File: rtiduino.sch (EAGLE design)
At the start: 144 parts, among them J1 DCJ0202, J2 3.5MM-JACK, J3 2.5MM-JACKPRO, J4 USB PROG, Q2 16MHz, U1 ATMEGA2560AU, U10 AQV252G, U11 AQV252G, U12 AQV252G, U13 AQV252G, U14 AQV252G, U15 AQV252G, U16 AQV252G, U17 AQV252G, U2 FT232RL, U20 AQV252G, U21 AQV252G, U22 AQV252G, U23 AQV252G, U24 AQV252G, U25 AQV252G, U26 AQV252G, U27 AQV252G, U3 LM2594HVM-5.0, U30 AQV252G, U31 AQV252G, U32 AQV252G, U33 AQV252G, U34 AQV252G, U35 AQV252G, U36 AQV252G, U37 AQV252G, U4 FT232RL, U5 FOD852, U6 LED-DRIVER, U7 FOD852

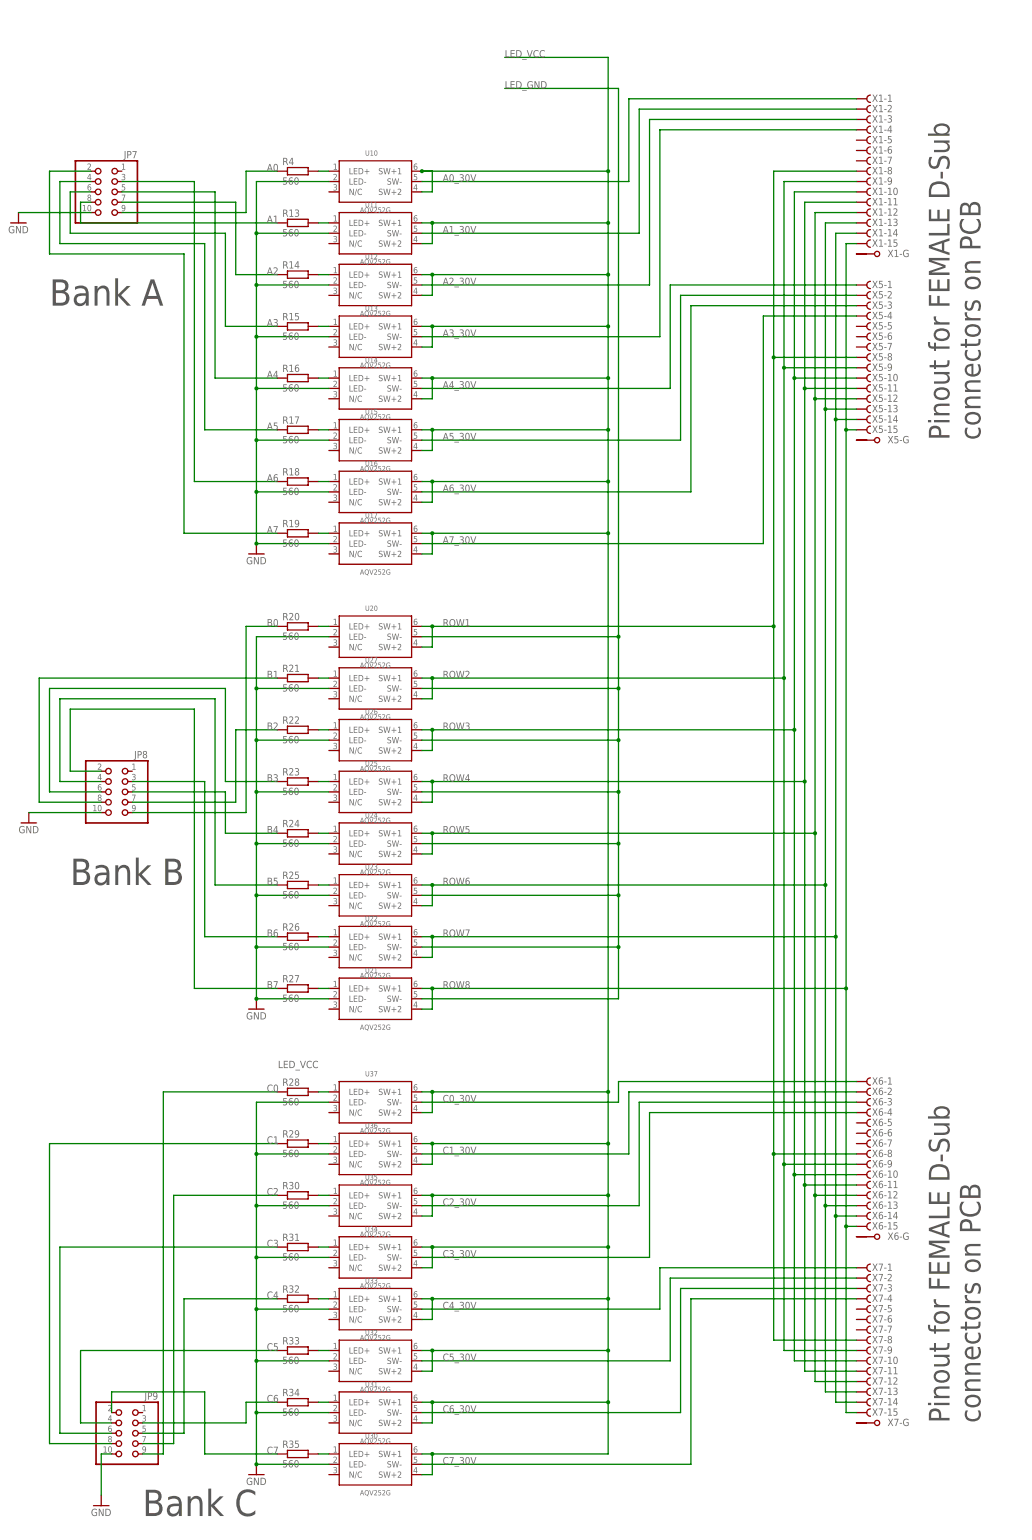
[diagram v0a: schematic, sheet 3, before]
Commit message: UPDATES
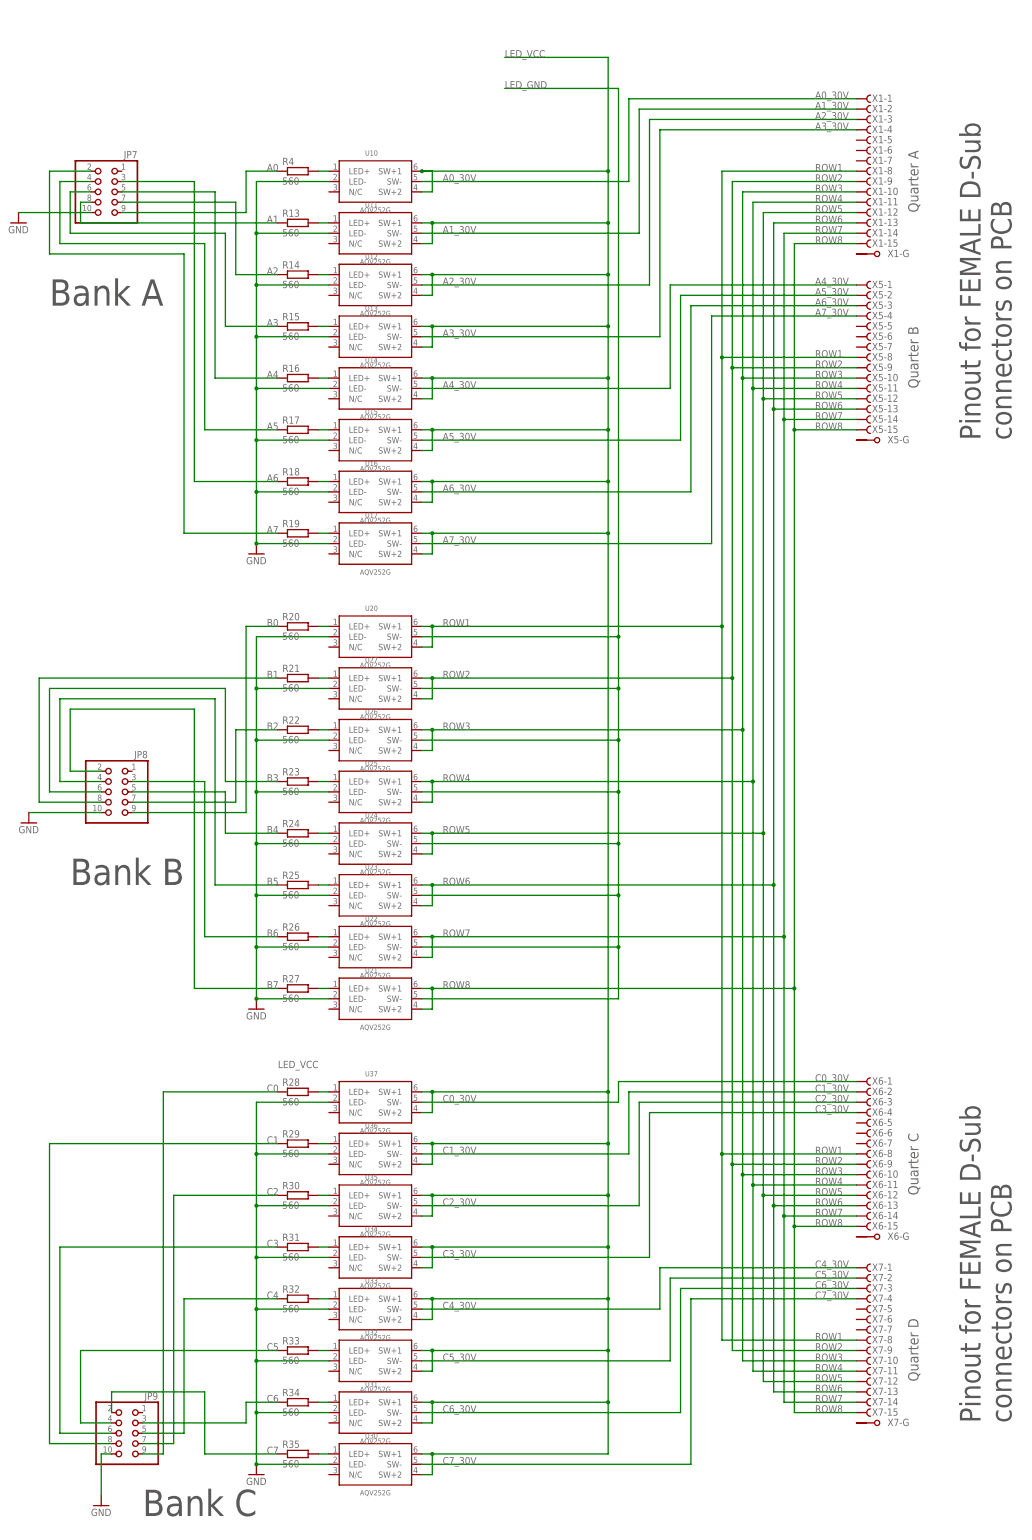
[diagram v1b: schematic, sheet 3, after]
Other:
- note added: "Quarter A"
- note added: "Quarter B"
- note added: "Quarter C"
- note added: "Quarter D"
